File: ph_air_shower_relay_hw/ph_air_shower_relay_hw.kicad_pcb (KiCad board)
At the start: 2 copper layers, 105.7 x 111.3 mm, 27 parts, among them J1 Conn_01x02, J2 Conn_01x02, J3 Conn_01x02, J4 Conn_01x10, J5 Conn_01x02, J6 Conn_01x07

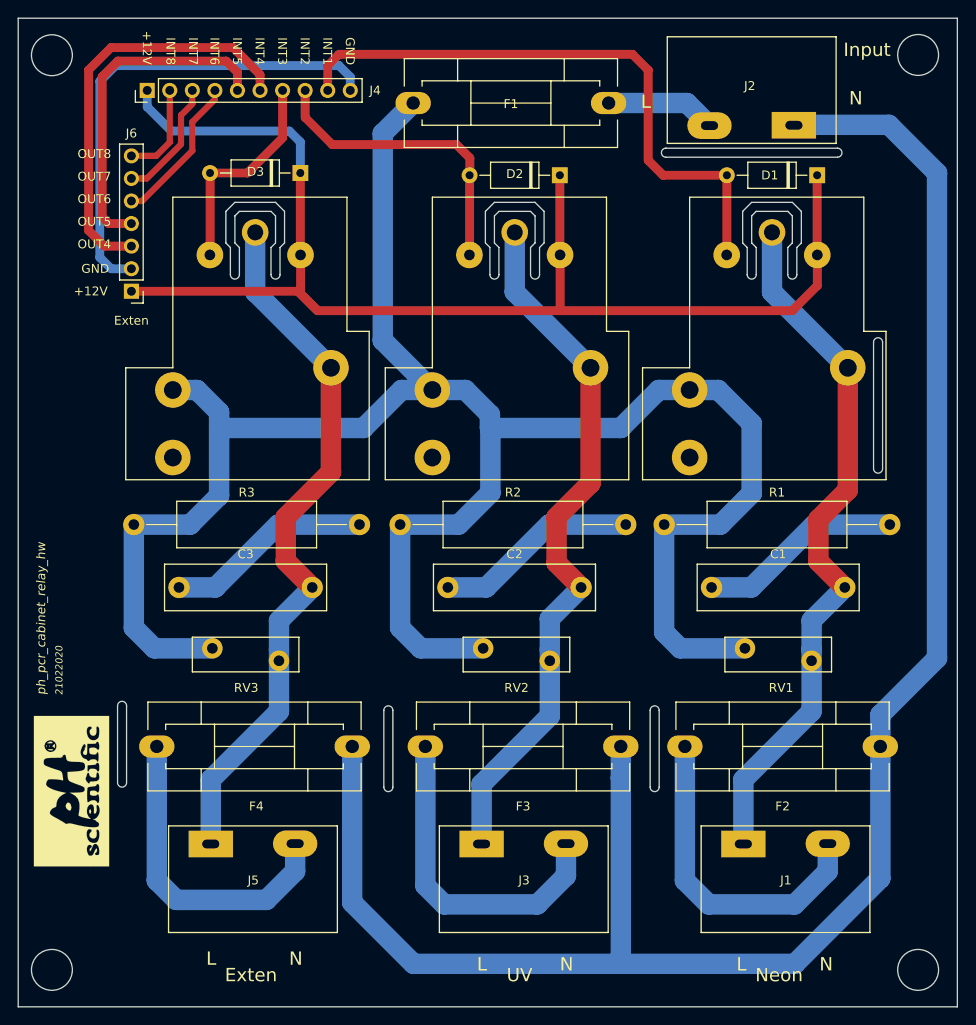
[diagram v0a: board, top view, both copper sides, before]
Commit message: Update Board Relay
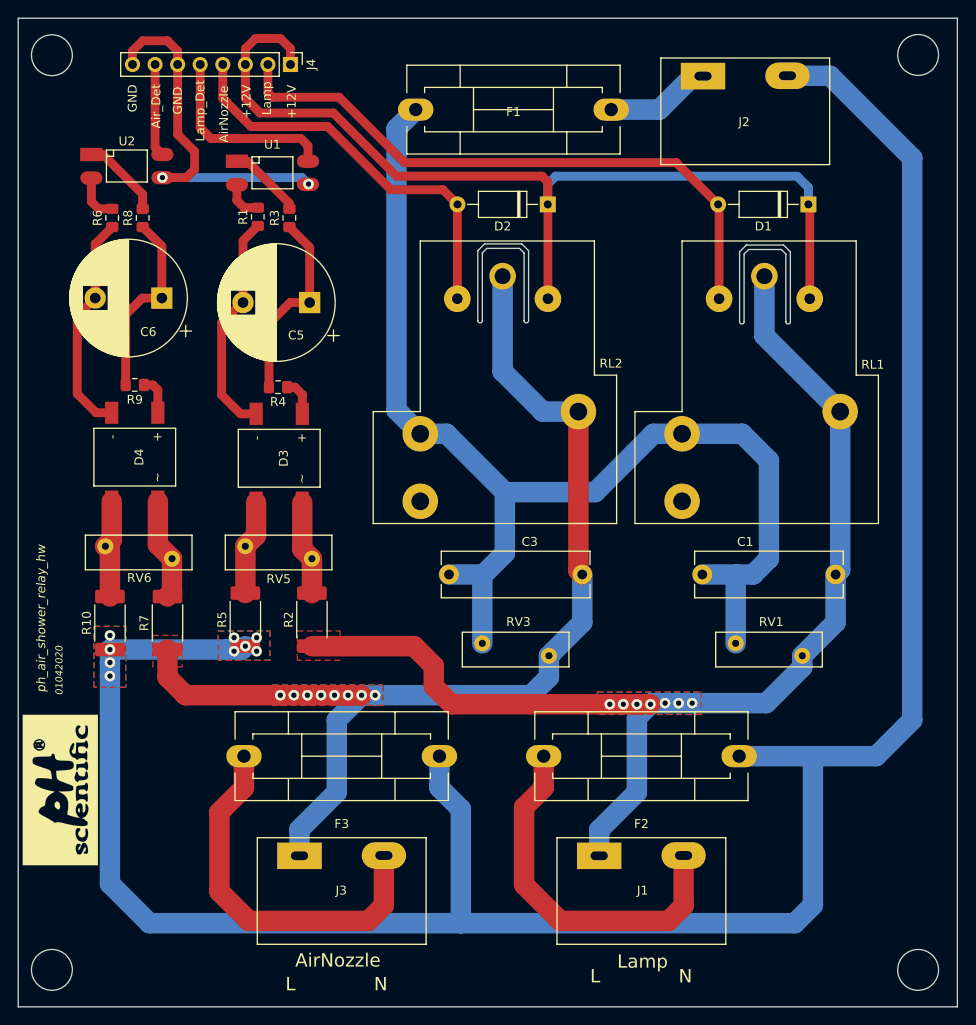
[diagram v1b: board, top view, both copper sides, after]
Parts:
- removed C2: 103J, Capacitor_THT:C_Rect_L18.0mm_W5.0mm_P15.00mm_FKS3_FKP3
- removed F4: Fuse, nhantt-kicad-lib:Fuseholder5x20_horiz_SemiClosed_Casing10x25mm
- removed the G*** at (131.0, 123.4) (x2)
- removed J5: Conn_01x02, nhantt-kicad-lib:Terminal-2P-9.5mm
- removed J6: Conn_01x07, Connector_PinHeader_2.54mm:PinHeader_1x07_P2.54mm_Vertical
- removed RL3: SLA-24VDC-SL-C, nhantt-kicad-lib:SLA-24VDC-SL-C
- removed RV2: Varistor, Varistor:RV_Disc_D12mm_W3.9mm_P7.5mm
- added C5: CP, Capacitors_THT:CP_Radial_D13.0mm_P7.50mm, F.Cu at (157.8, 68.4)
- added C6: CP, Capacitors_THT:CP_Radial_D13.0mm_P7.50mm, F.Cu at (141.1, 67.9)
- added D4: Bridge_Diode, vinhtho_lib:DB107S, F.Cu at (138.1, 85.8)
- added G***: LOGO, PH_Footprint:logo, F.Cu at (129.7, 123.3)
- added G***: LOGO, PH_Footprint:logo, B.Cu at (129.7, 123.3)
- added R10: 220K/1/2w, Resistor_SMD:R_2512_6332Metric_Pad1.52x3.35mm_HandSolder, F.Cu at (135.3, 104.5)
- added R4: 390K, Resistor_SMD:R_0805_2012Metric_Pad1.15x1.40mm_HandSolder, F.Cu at (154.2, 77.9)
- added R5: 220K/1/2w, Resistor_SMD:R_2512_6332Metric_Pad1.52x3.35mm_HandSolder, F.Cu at (150.5, 104.1)
- added R6: 1K, Resistor_SMD:R_0805_2012Metric_Pad1.15x1.40mm_HandSolder, F.Cu at (135.5, 58.9)
- added R7: 220K/1/2w, Resistor_SMD:R_2512_6332Metric_Pad1.52x3.35mm_HandSolder, F.Cu at (141.8, 104.5)
- added R8: 1K, Resistor_SMD:R_0805_2012Metric_Pad1.15x1.40mm_HandSolder, F.Cu at (139.0, 58.9)
- added R9: 390K, Resistor_SMD:R_0805_2012Metric_Pad1.15x1.40mm_HandSolder, F.Cu at (138.1, 77.7)
- added RV5: Varistor, Varistor:RV_Disc_D12mm_W3.9mm_P7.5mm, F.Cu at (158.0, 97.2)
- added RV6: Varistor, Varistor:RV_Disc_D12mm_W3.9mm_P7.5mm, F.Cu at (142.3, 97.2)
- added U1: PC817, vinhtho_lib:Optocoupler_SMD, F.Cu at (153.6, 53.8)
- added U2: PC817, vinhtho_lib:Optocoupler_SMD, F.Cu at (137.2, 53.0)
- C1, C3: value 103J -> 152; footprint Capacitor_THT:C_Rect_L18.0mm_W5.0mm_P15.00mm_FKS3_FKP3 -> Capacitors_THT:C_Rect_L16.5mm_W5.0mm_P15.00mm_MKT
- D3: value FR107 -> Bridge_Diode; footprint Diode_THT:D_A-405_P10.16mm_Horizontal -> vinhtho_lib:DB107S
- F1, F2, F3: footprint nhantt-kicad-lib:Fuseholder5x20_horiz_SemiClosed_Casing10x25mm -> vinhtho_lib:Fuseholder5x20_horiz_SemiClosed_Casing10x25mm
- J1, J2, J3: footprint nhantt-kicad-lib:Terminal-2P-9.5mm -> vinhtho_lib:Terminal-2P-9.5mm
- J4: value Conn_01x10 -> Conn_01x08; footprint Connector_PinHeader_2.54mm:PinHeader_1x10_P2.54mm_Vertical -> Connector_PinHeader_2.54mm:PinHeader_1x08_P2.54mm_Vertical
- R1, R3: value 220R -> 1K; footprint Resistor_THT:R_Axial_DIN0516_L15.5mm_D5.0mm_P25.40mm_Horizontal -> Resistor_SMD:R_0805_2012Metric_Pad1.15x1.40mm_HandSolder
- R2: value 220R -> 220K/1/2w; footprint Resistor_THT:R_Axial_DIN0516_L15.5mm_D5.0mm_P25.40mm_Horizontal -> Resistor_SMD:R_2512_6332Metric_Pad1.52x3.35mm_HandSolder
- RL1, RL2: footprint nhantt-kicad-lib:SLA-24VDC-SL-C -> vinhtho_lib:SLA-24VDC-SL-C
- moved R1 57.4 mm to (151.9, 58.8), turned to 90 degrees
- moved R3 38.7 mm to (155.5, 58.9), turned to 90 degrees
- moved D3 32.2 mm to (154.3, 85.9), turned to 90 degrees
- moved C3 30.4 mm to (173.4, 99.0)
- moved RV3 30.4 mm to (177.2, 106.8)
- moved J3 20.5 mm to (161.4, 130.6)
- moved F3 20.4 mm to (172.4, 119.5)
- moved J4 16.4 mm to (155.6, 41.6), turned to 270 degrees
- moved J1 16.3 mm to (195.1, 130.6)
- moved F2 15.9 mm to (206.1, 119.5)
- moved R2 14.6 mm to (158.0, 104.1), turned to 90 degrees
- moved J2 5.66 mm to (206.8, 42.9), turned to 0 degrees
- moved RL2 5.11 mm to (179.5, 78.6)
- moved RL1 5.00 mm to (208.9, 78.6)
- moved D2 3.55 mm to (184.6, 57.4)
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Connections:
- C1 pad 1: Net-(C1-Pad1) -> /L
- C1 pad 2: Net-(C1-Pad2) -> /L1
- C3 pad 1: Net-(C3-Pad1) -> /L
- C3 pad 2: Net-(C3-Pad2) -> /L2
- D1 pad 1: +24V -> +12V
- D1 pad 2: /RL1 -> /RELAY1
- D2 pad 1: +24V -> +12V
- D2 pad 2: /RL2 -> /RELAY2
- D3 pad 1: +24V -> Net-(D3-Pad1)
- D3 pad 2: /RL3 -> Net-(D3-Pad2)
- J1 pad 1: Net-(C1-Pad2) -> /L1
- J2 pad 1: /N -> Net-(F1-Pad2)
- J2 pad 2: Net-(F1-Pad2) -> /N
- J3 pad 1: Net-(C2-Pad2) -> /L2
- J4 pad 1: +24V -> +12V
- J4 pad 2: /INT8 -> /RELAY1
- J4 pad 3: /INT7 -> +12V
- J4 pad 4: /INT6 -> /RELAY2
- J4 pad 5: /INT5 -> /LAMP_DET
- J4 pad 6: /INT4 -> GND
- J4 pad 7: /RL3 -> /AIR_DET
- J4 pad 8: /RL2 -> GND
- R1 pad 1: /L -> Net-(C5-Pad2)
- R1 pad 2: Net-(C1-Pad1) -> Net-(R1-Pad2)
- R2 pad 1: /L -> /L1
- R2 pad 2: Net-(C2-Pad1) -> Net-(D3-Pad3)
- R3 pad 1: /L -> Net-(C5-Pad1)
- R3 pad 2: Net-(C3-Pad1) -> Net-(R3-Pad2)
- RL1 pad 1: /RL1 -> /RELAY1
- RL1 pad 2: Net-(C1-Pad2) -> /L1
- RL1 pad 3: +24V -> +12V
- RL1 pad 4: Net-(C1-Pad2) -> /L1
- RL2 pad 1: /RL2 -> /RELAY2
- RL2 pad 2: Net-(C2-Pad2) -> /L2
- RL2 pad 3: +24V -> +12V
- RL2 pad 4: Net-(C2-Pad2) -> /L2
- RV1 pad 2: Net-(C1-Pad2) -> /L1
- RV3 pad 2: Net-(C3-Pad2) -> /L2
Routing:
- net +24V: track 147.2 -> 0.00 mm
- net /L1: track 0.00 -> 129.7 mm, vias 0 -> 7
- net /L2: track 0.00 -> 121.4 mm, vias 0 -> 8
- net +12V: track 0.00 -> 109.6 mm
- net /L: track 233.9 -> 133.4 mm
- net Net-(C3-Pad2): track 80.4 -> 0.00 mm
- net Net-(C2-Pad2): track 79.7 -> 0.00 mm
- net Net-(C1-Pad2): track 79.7 -> 0.00 mm
- net /RELAY1: track 0.00 -> 69.7 mm
- net /RL1: track 68.8 -> 0.00 mm
- net /N: track 208.3 -> 262.4 mm, vias 0 -> 9
- net /INT4: track 47.0 -> 0.00 mm
- net /RELAY2: track 0.00 -> 45.8 mm
- net /INT5: track 37.9 -> 0.00 mm
- net Net-(F4-Pad2): track 36.0 -> 0.00 mm
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- added copper zone on B.Cu, net /L1
- added copper zone on F.Cu, net /L1
- added copper zone on B.Cu, net /L2
- added copper zone on F.Cu, net /L2
- added copper zone on B.Cu, net /N
- added copper zone on F.Cu, net /N
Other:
- outline, holes or cut-outs redrawn
- board text added: "01042020"
- board text added: "AirNozzle"
- board text added: "Air_Det"
- board text added: "Lamp"
- board text added: "Lamp_Det"
- board text added: "ph_air_shower_relay_hw"
- board text removed: "21022020"
- board text removed: "Exten"
- board text removed: "INT1"
- board text removed: "INT2"
- board text removed: "INT3"
- board text removed: "INT4"
- board text removed: "INT5"
- board text removed: "INT6"
- board text removed: "INT7"
- board text removed: "INT8"
- board text removed: "Input"
- board text removed: "Neon"
- board text removed: "OUT4"
- board text removed: "OUT5"
- board text removed: "OUT6"
- board text removed: "OUT7"
- board text removed: "OUT8"
- board text removed: "UV"
- board text removed: "ph_pcr_cabinet_relay_hw"
